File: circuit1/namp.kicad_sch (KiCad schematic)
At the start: 97 parts, among them J1 Screw_Terminal_01x08, J2 Screw_Terminal_01x04, J3 Screw_Terminal_01x04, J4 Conn_01x08_Female, U1 NRF52840-DONGLE, U2 MCP6004, U3 MCP6004, U4 MCP1501-33xSN, U5 MCP3564, U6 MCP1754S-5002xCB, U7 MCP1754S-5002xCB, U8 MCP1754S-3302xCB

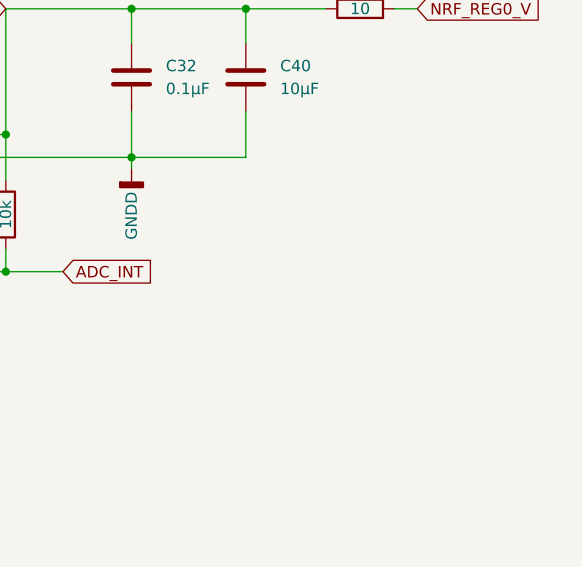
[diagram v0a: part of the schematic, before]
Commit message: update
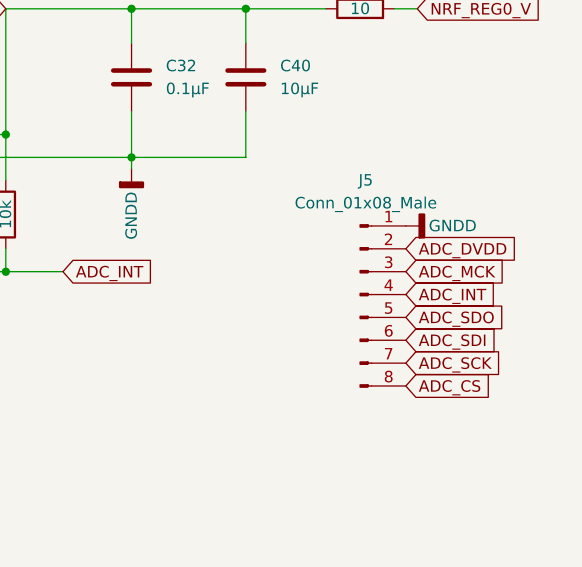
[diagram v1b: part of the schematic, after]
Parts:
- added J5: Conn_01x08_Male, Connector_PinHeader_2.54mm:PinHeader_1x08_P2.54mm_Vertical, symbol Connector:Conn_01x08_Male
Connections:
- net ADC_CS: now also J5.8 (Pin_8)
- net ADC_DVDD: now also J5.2 (Pin_2)
- net ADC_INT: now also J5.4 (Pin_4)
- net ADC_MCK: now also J5.3 (Pin_3)
- net ADC_SCK: now also J5.7 (Pin_7)
- net ADC_SDI: now also J5.6 (Pin_6)
- net ADC_SDO: now also J5.5 (Pin_5)
- net GND: now also J5.1 (Pin_1)
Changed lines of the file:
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@@
+    )
+  )
+  (global_label "ADC_SCK" (shape input) (at 560.07 290.83 0) (fields_autoplaced)
+    (effects (font (size 1.27 1.27)) (justify left))
+    (property "Intersheet References" "${INTERSHEET_REFS}" (id 0) (at 570.8288 290.7506 0)
+      (effects (font (size 1.27 1.27)) (justify left) hide)
     )
   )
@@
     )
   )
+  (global_label "ADC_MCK" (shape input) (at 560.07 280.67 0) (fields_autoplaced)
+    (effects (font (size 1.27 1.27)) (justify left))
+    (property "Intersheet References" "${INTERSHEET_REFS}" (id 0) (at 571.0707 280.5906 0)
+      (effects (font (size 1.27 1.27)) (justify left) hide)
+    )
+  )
   (global_label "ADC_INT" (shape input) (at 234.95 123.19 0) (fields_autoplaced)
     (effects (font (size 1.27 1.27)) (justify left))
@@
     )
   )
+  (global_label "ADC_CS" (shape input) (at 560.07 293.37 0) (fields_autoplaced)
+    (effects (font (size 1.27 1.27)) (justify left))
+    (property "Intersheet References" "${INTERSHEET_REFS}" (id 0) (at 569.5588 293.2906 0)
+      (effects (font (size 1.27 1.27)) (justify left) hide)
+    )
+  )
+  (global_label "ADC_INT" (shape input) (at 560.07 283.21 0) (fields_autoplaced)
+    (effects (font (size 1.27 1.27)) (justify left))
+    (property "Intersheet References" "${INTERSHEET_REFS}" (id 0) (at 569.9821 283.1306 0)
+      (effects (font (size 1.27 1.27)) (justify left) hide)
+    )
+  )
+  (global_label "ADC_SDO" (shape input) (at 560.07 285.75 0) (fields_autoplaced)
+    (effects (font (size 1.27 1.27)) (justify left))
+    (property "Intersheet References" "${INTERSHEET_REFS}" (id 0) (at 570.8893 285.6706 0)
+      (effects (font (size 1.27 1.27)) (justify left) hide)
+    )
+  )
   (global_label "TIA1_V" (shape input) (at 30.48 317.5 180) (fields_autoplaced)
     (effects (font (size 1.27 1.27)) (justify right))
@@
     )
   )
+  (global_label "ADC_SDI" (shape input) (at 560.07 288.29 0) (fields_autoplaced)
+    (effects (font (size 1.27 1.27)) (justify left))
+    (property "Intersheet References" "${INTERSHEET_REFS}" (id 0) (at 570.1636 288.2106 0)
+      (effects (font (size 1.27 1.27)) (justify left) hide)
+    )
+  )
   (global_label "ADC_SDO" (shape input) (at 234.95 125.73 0) (fields_autoplaced)
     (effects (font (size 1.27 1.27)) (justify left))
@@
     (effects (font (size 1.27 1.27)) (justify left))
     (property "Intersheet References" "${INTERSHEET_REFS}" (id 0) (at 244.4388 133.2706 0)
+      (effects (font (size 1.27 1.27)) (justify left) hide)
+    )
+  )
+  (global_label "ADC_DVDD" (shape input) (at 560.07 278.13 0) (fields_autoplaced)
+    (effects (font (size 1.27 1.27)) (justify left))
+    (property "Intersheet References" "${INTERSHEET_REFS}" (id 0) (at 571.9779 278.2094 0)
       (effects (font (size 1.27 1.27)) (justify left) hide)
     )
@@
     (pin "1")
   )
+  (symbol (lib_id "Connector:Conn_01x08_Male") (at 554.99 283.21 0) (unit 1)
+    (in_bom yes) (on_board yes) (fields_autoplaced)
+    (property "Reference" "J5" (id 0) (at 555.625 270.51 0))
+    (property "Value" "Conn_01x08_Male" (id 1) (at 555.625 273.05 0))
+    (property "Footprint" "Connector_PinHeader_2.54mm:PinHeader_1x08_P2.54mm_Vertical" (id 2) (at 554.99 283.21 0)
+      (effects (font (size 1.27 1.27)) hide)
+    )
+    (property "Datasheet" "~" (id 3) (at 554.99 283.21 0)
+      (effects (font (size 1.27 1.27)) hide)
+    )
+    (pin "1")
+    (pin "2")
+    (pin "3")
+    (pin "4")
+    (pin "5")
+    (pin "6")
+    (pin "7")
+    (pin "8")
+  )
   (symbol (lib_id "Device:R") (at 77.47 187.96 270) (unit 1)
     (in_bom yes) (on_board yes)
@@
     (pin "13")
     (pin "14")
+  )
+  (symbol (lib_id "power:GNDD") (at 560.07 275.59 90) (unit 1)
+    (in_bom yes) (on_board yes)
+    (property "Reference" "#PWR0115" (id 0) (at 566.42 275.59 0)
+      (effects (font (size 1.27 1.27)) hide)
+    )
+    (property "Value" "GNDD" (id 1) (at 562.61 275.59 90)
+      (effects (font (size 1.27 1.27)) (justify right))
+    )
+    (property "Footprint" "" (id 2) (at 560.07 275.59 0)
+      (effects (font (size 1.27 1.27)) hide)
+    )
+    (property "Datasheet" "" (id 3) (at 560.07 275.59 0)
+      (effects (font (size 1.27 1.27)) hide)
+    )
+    (pin "1")
   )
   (symbol (lib_id "power:GNDD") (at 163.83 381 0) (unit 1)
@@
       (reference "#PWR0114") (unit 1) (value "GNDD") (footprint "")
     )
+    (path "/34238737-e2f4-4660-8dc4-f6374bb15abf"
+      (reference "#PWR0115") (unit 1) (value "GNDD") (footprint "")
+    )
     (path "/1f7471b5-dfd9-4156-b85a-3ecaede73fff"
       (reference "#PWR0116") (unit 1) (value "GNDA") (footprint "")
@@
       (reference "J4") (unit 1) (value "Conn_01x08_Female") (footprint "Connector_PinHeader_2.54mm:PinHeader_1x08_P2.54mm_Vertical")
     )
+    (path "/1763f786-dd71-4840-968a-c65e7d3470b9"
+      (reference "J5") (unit 1) (value "Conn_01x08_Male") (footprint "Connector_PinHeader_2.54mm:PinHeader_1x08_P2.54mm_Vertical")
+    )
     (path "/0a4670fe-f411-47c9-8912-2ac7b841eb8f"
